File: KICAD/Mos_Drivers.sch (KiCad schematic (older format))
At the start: 16 parts, among them U12 UCC27284-Q1

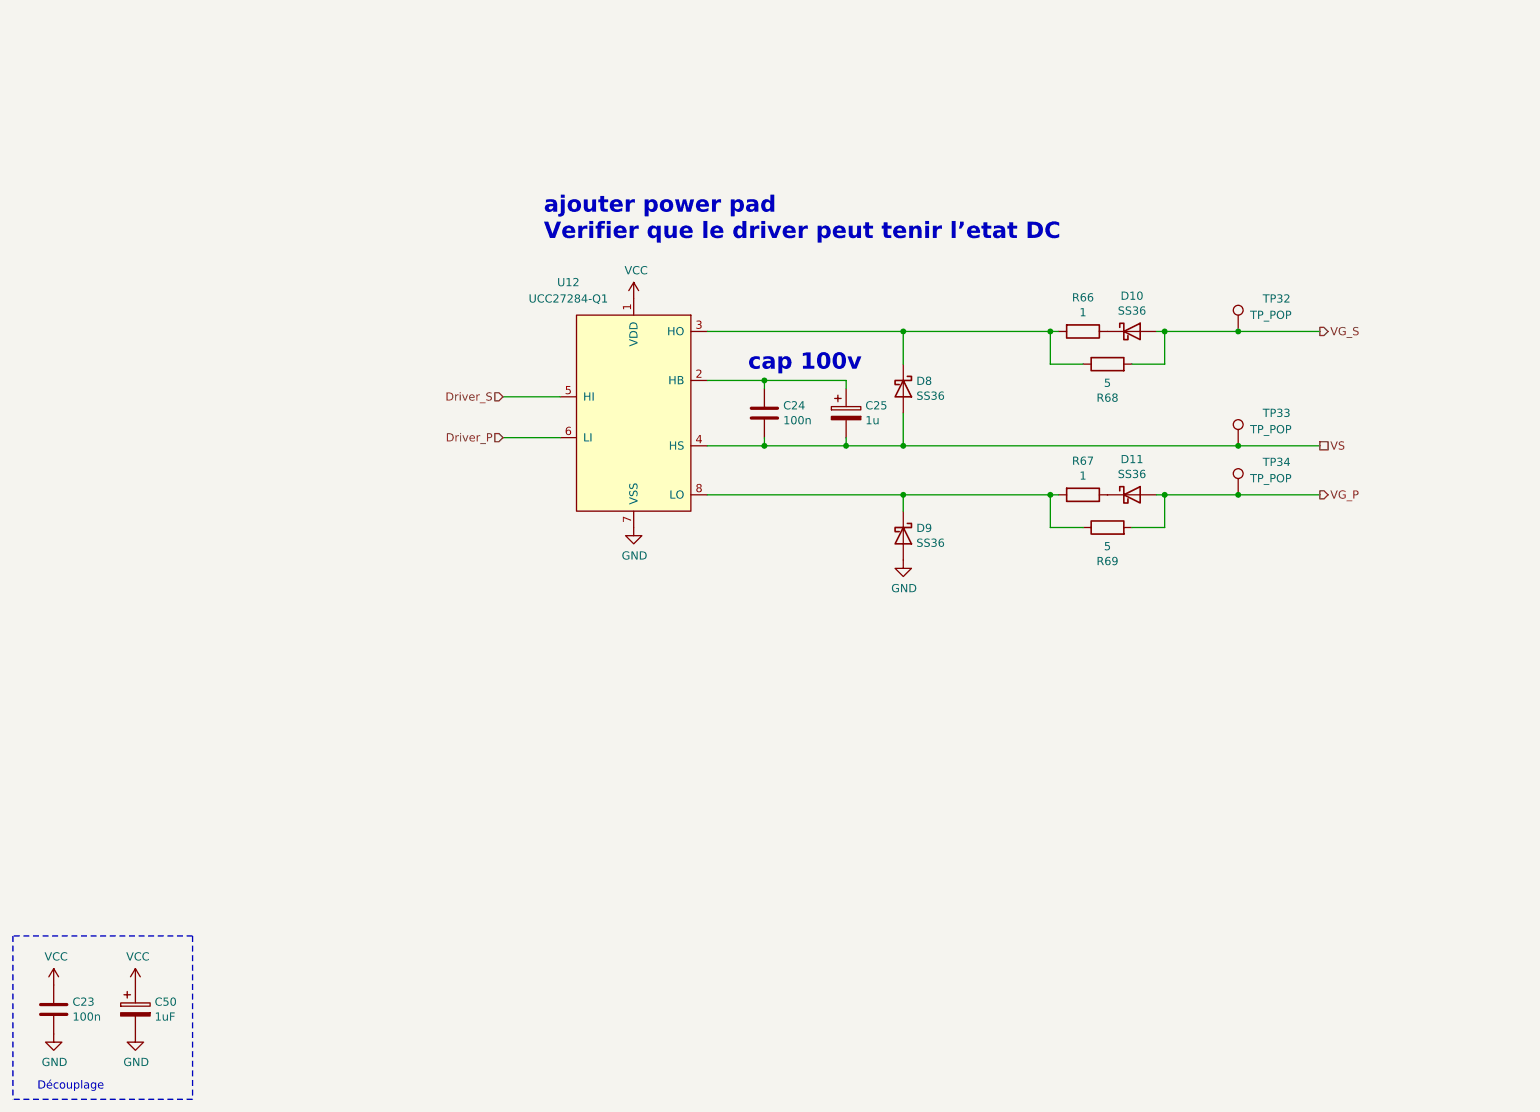
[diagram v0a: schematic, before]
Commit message: cleanup silkscreen
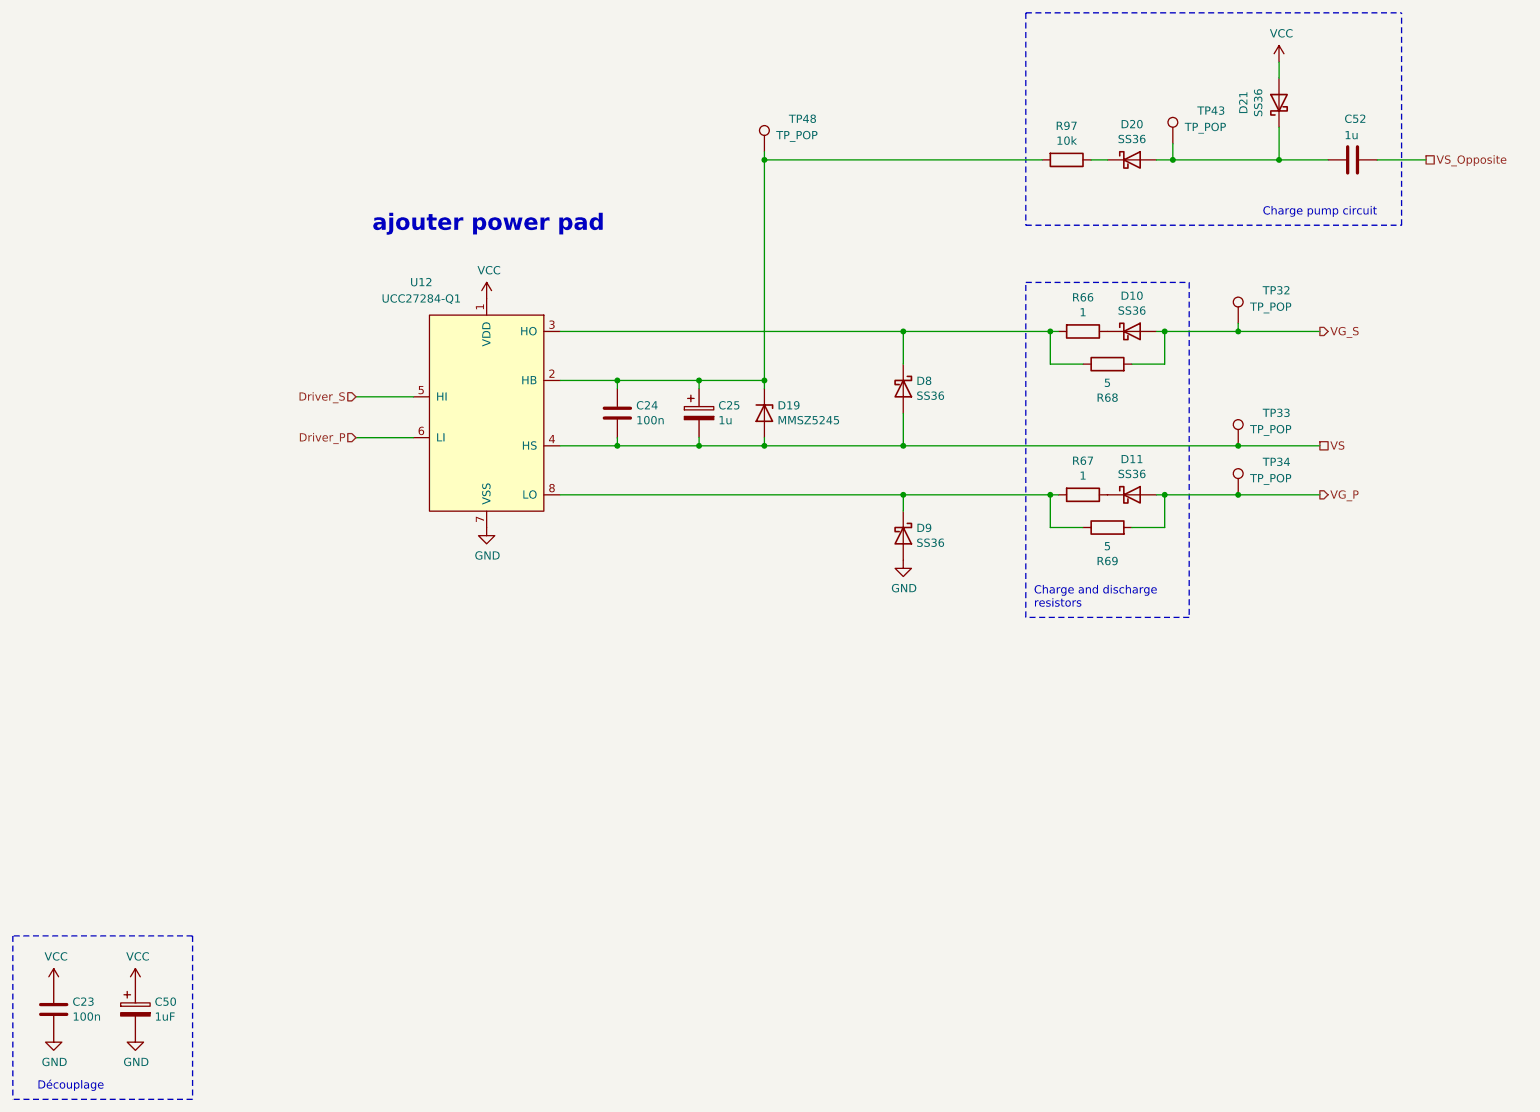
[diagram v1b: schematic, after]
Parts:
- added C52: 1u, Sesame_footprint:C_0805_2012Metric_Pad1.18x1.45mm_HandSolder, symbol Device:C
- added D19: MMSZ5245, Diode_SMD:D_SOD-123, symbol Device:D_Zener
- added D20, D21: SS36, Diode_SMD:D_SMA_Handsoldering, symbol Device:D_Schottky
- added R97: 10k, Sesame_footprint:R_0805_2012Metric_Pad1.20x1.40mm_HandSolder, symbol Device:R
- added TP43, TP48: TP_POP, TestPoint:TestPoint_Loop_D1.80mm_Drill1.0mm_Beaded, symbol Connector:TestPoint
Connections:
- net VCC: now also D21.2 (A)
- net VS: now also D19.2 (A)
- net at C24.1, C25.1, U12.2 (HB): now also D19.1 (K), R97.2, TP48.1
- new net: C52.2, D20.2 (A), D21.1 (K), TP43.1
- new net: D20.1 (K), R97.1
- new net VS_Opposite: C52.1
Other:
- note added: "Charge and discharge\nresistors"
- note added: "Charge pump circuit"
- note added: "ajouter power pad"
- note removed: "ajouter power pad\nVerifier que le driver peut tenir l’etat DC"
- note removed: "cap 100v"
- moved on the sheet: C24, C25, TP32, U12
